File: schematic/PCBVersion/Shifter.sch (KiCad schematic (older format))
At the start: 10 parts, among them U19 74LS157, U20 74LS157, U21 74LS157, U22 74LS157, U23 74LS157, U24 74LS157, U25 74LS157, U26 74LS157, U27 74LS157, U28 74LS157

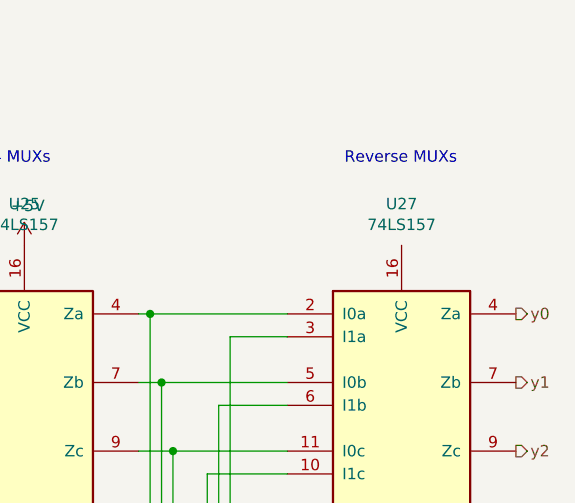
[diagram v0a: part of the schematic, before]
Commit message: pcbVersion: regset + alu
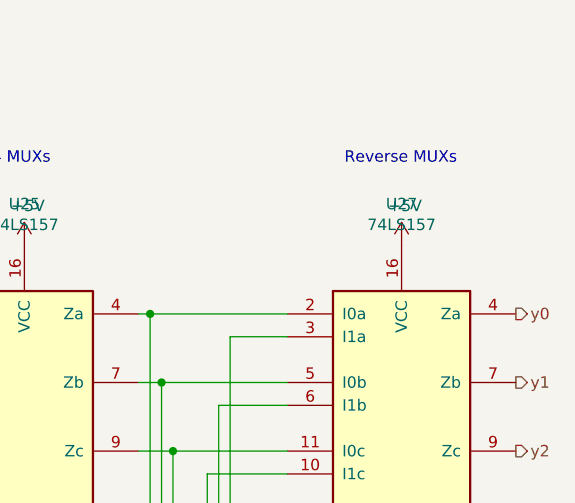
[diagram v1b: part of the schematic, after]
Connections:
- net +5V: now also U27.16 (VCC)
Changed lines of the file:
@@
 $Descr A4 11693 8268
 encoding utf-8
-Sheet 13 13
+Sheet 3 14
 Title ""
 Date ""
@@
 Wire Wire Line
 	7650 5300 8050 5300
+$Comp
+L power:+5V #PWR0108
+U 1 1 6032FB0C
+P 8800 1900
+F 0 "#PWR0108" H 8800 1750 50  0001 C CNN
+F 1 "+5V" H 8815 2073 50  0000 C CNN
+F 2 "" H 8800 1900 50  0001 C CNN
+F 3 "" H 8800 1900 50  0001 C CNN
+	1    8800 1900
+	1    0    0    -1
+$EndComp
 $EndSCHEMATC
